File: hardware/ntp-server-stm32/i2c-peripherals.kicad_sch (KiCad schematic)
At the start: 13 parts, among them U57 TMP117xxDRV, U58 TMP117xxDRV, U59 LIS2DH12TR, U60 ATECC608B-SSHDA, U61 IIS2MDCTR

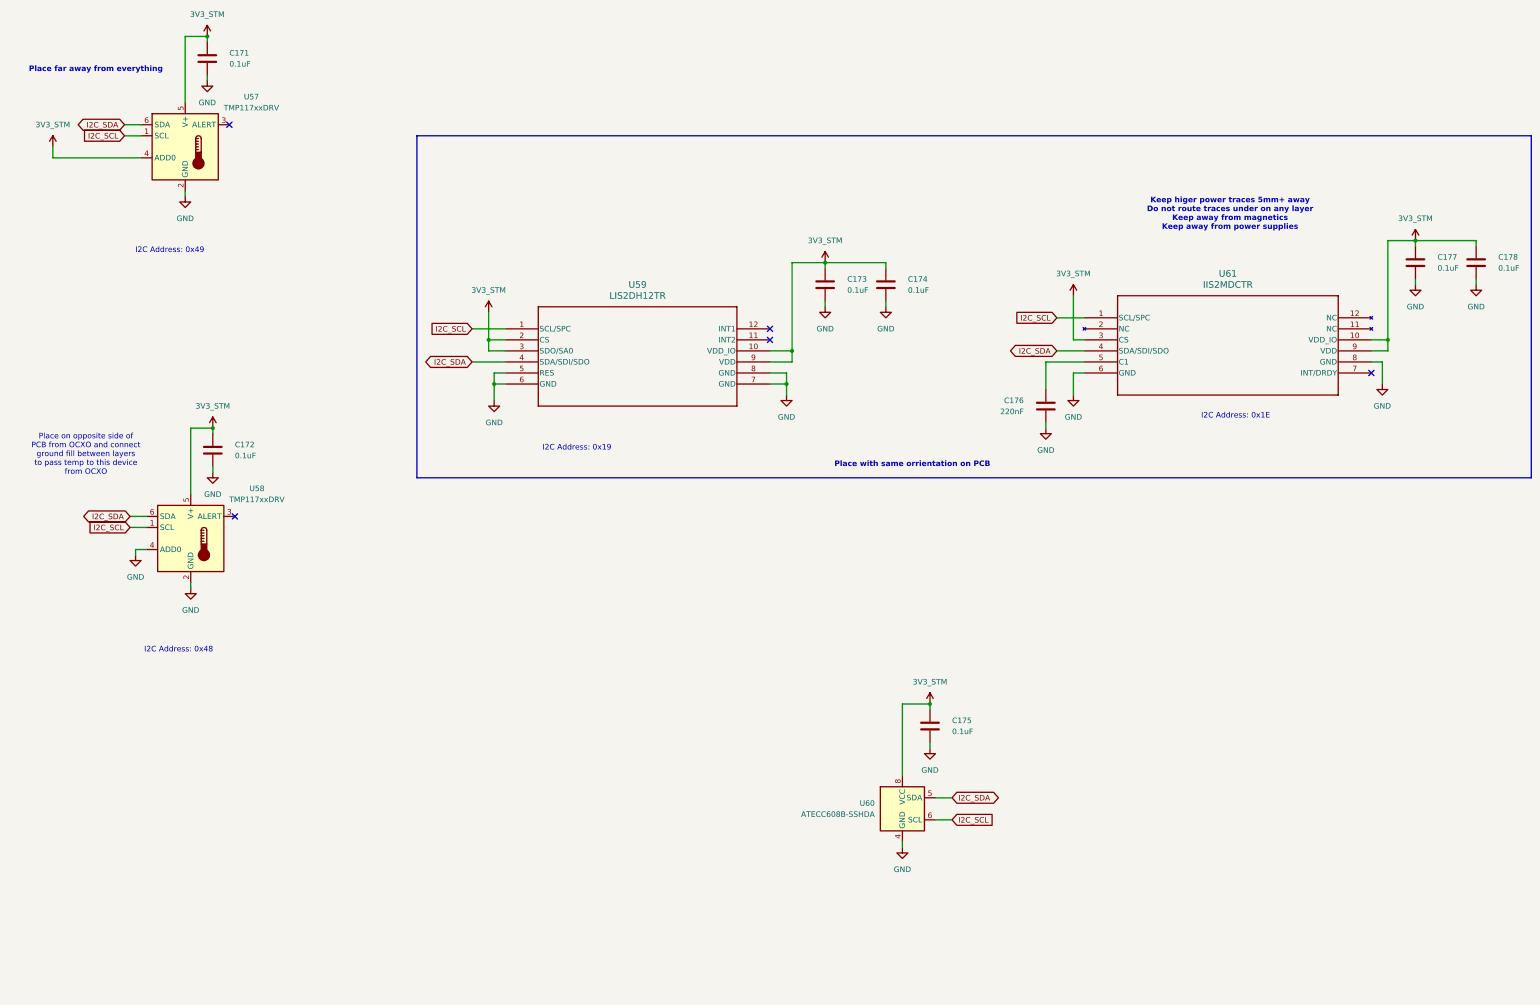
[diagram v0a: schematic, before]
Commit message: Updates
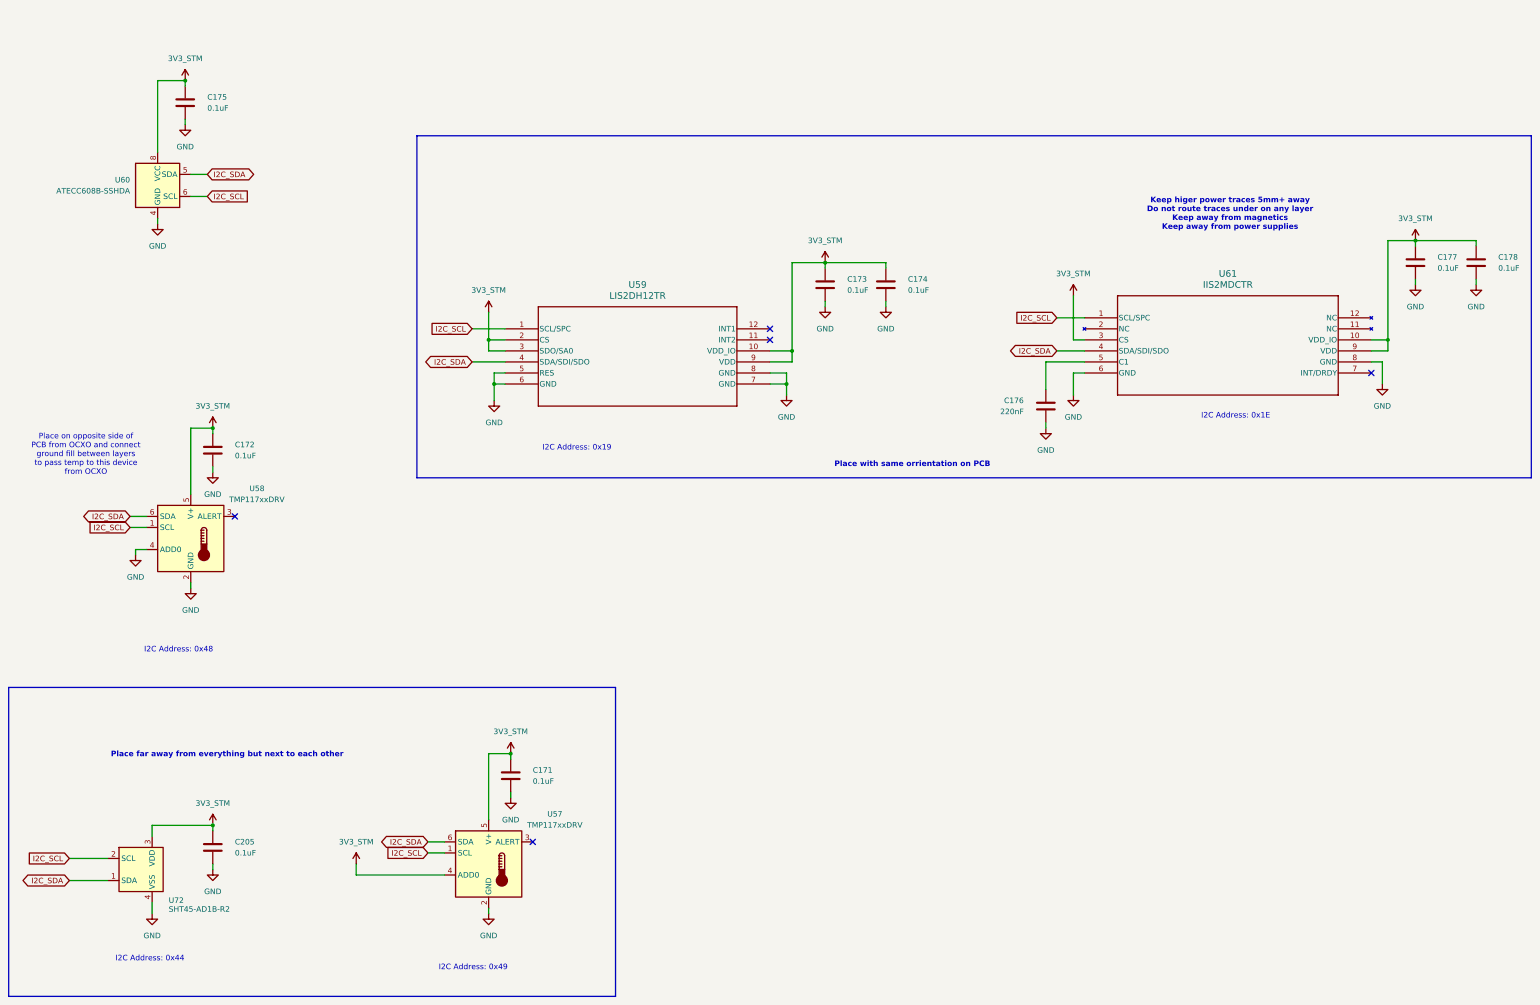
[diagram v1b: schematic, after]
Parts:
- added C205: 0.1uF, 0402 (1005 Metric), symbol Device:C
- added U72: SHT45-AD1B-R2, Sensor_Humidity:Sensirion_DFN-4_1.5x1.5mm_P0.8mm_SHT4x_NoCentralPad, symbol Sensor_Humidity:SHT4x
- C171, C172, C173, C174, C175, C177, C178: footprint C_0402_1005Metric -> 0402 (1005 Metric); DIELECTRIC (none) -> X7R; DIGIKEY_PART_NUMBER 490-6328-2-ND -> 490-4759-1-ND; MANUFACTURER_PART_NUMBER GRM155R71C104KA88J -> GCM155R71C104KA55D; TOLERANCE (none) -> 10%; VOLTAGE (none) -> 16V
- C176: footprint C_0402_1005Metric -> 0402 (1005 Metric); DIELECTRIC (none) -> X7R; DIGIKEY_PART_NUMBER 445-5972-1-ND -> 490-GCM155R71C224KE02JCT-ND; MANUFACTURER TDK -> Murata; MANUFACTURER_PART_NUMBER C2012X7R1E475K125AB -> GCM155R71C224KE02J; TOLERANCE (none) -> 10%; VOLTAGE (none) -> 16V
- U57, U58: MANUFACTURER (none) -> Texas Instruments; MANUFACTURER_PART_NUMBER TMP117xxDRV -> TMP117AIDRVR
- U59, U61: MANUFACTURER (none) -> STMicroelectronics
- U60: MANUFACTURER (none) -> Microchip
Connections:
- net 3V3_STM: now also C205.1, U72.3 (VDD)
- net GND: now also C205.2, U72.4 (VSS)
- net I2C_SCL: now also U72.2 (SCL)
- net I2C_SDA: now also U72.1 (SDA)
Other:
- note added: "I2C Address: 0x44"
- note added: "Place far away from everything but next to each other"
- note removed: "Place far away from everything"
- moved on the sheet: C171, C175, U57, U60

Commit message: Bom updates
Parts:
- U57, U58: DIGIKEY_PART_NUMBER (none) -> 296-51834-1-ND
- U59: DIGIKEY_PART_NUMBER (none) -> 497-14851-1-ND
- U60: DIGIKEY_PART_NUMBER (none) -> 150-ATECC608B-SSHDA-TCT-ND
- U61: DIGIKEY_PART_NUMBER (none) -> 497-17728-1-ND
- U72: DIGIKEY_PART_NUMBER (none) -> 1649-SHT45-AD1B-R2CT-ND
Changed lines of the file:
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@@
+			)
+		)
+		(property "DIGIKEY_PART_NUMBER" "296-51834-1-ND"
+			(at 148.59 224.79 0)
+			(hide yes)
+			(show_name no)
+			(do_not_autoplace no)
+			(effects
+				(font
+					(size 1.27 1.27)
+				)
 			)
 		)
@@
 			)
 		)
+		(property "DIGIKEY_PART_NUMBER" "497-14851-1-ND"
+			(at 152.4 101.6 0)
+			(hide yes)
+			(show_name no)
+			(do_not_autoplace no)
+			(effects
+				(font
+					(size 1.27 1.27)
+				)
+			)
+		)
 		(pin "1"
 		)
@@
 			)
 		)
+		(property "DIGIKEY_PART_NUMBER" "1649-SHT45-AD1B-R2CT-ND"
+			(at 68.58 226.06 0)
+			(hide yes)
+			(show_name no)
+			(do_not_autoplace no)
+			(effects
+				(font
+					(size 1.27 1.27)
+				)
+			)
+		)
 		(pin "2"
 		)
@@
 			)
 		)
+		(property "DIGIKEY_PART_NUMBER" "497-17728-1-ND"
+			(at 285.75 99.06 0)
+			(hide yes)
+			(show_name no)
+			(do_not_autoplace no)
+			(effects
+				(font
+					(size 1.27 1.27)
+				)
+			)
+		)
 		(pin "4"
 		)
@@
 			)
 		)
+		(property "DIGIKEY_PART_NUMBER" "150-ATECC608B-SSHDA-TCT-ND"
+			(at 72.39 68.58 0)
+			(hide yes)
+			(show_name no)
+			(do_not_autoplace no)
+			(effects
+				(font
+					(size 1.27 1.27)
+				)
+			)
+		)
 		(pin "5"
 		)
@@
 			(hide yes)
 			(show_name no)
+			(do_not_autoplace no)
+			(effects
+				(font
+					(size 1.27 1.27)
+				)
+			)
+		)
+		(property "DIGIKEY_PART_NUMBER" "296-51834-1-ND"
+			(at 80.01 149.86 0)
+			(hide yes)
+			(show_name no)

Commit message: Bom updates
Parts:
- U59: footprint LGA-12_STM -> sts1000:LGA-12_STM
- U61: footprint LGA-12_2X2X0P7_STM -> sts1000:LGA-12_2X2X0P7_STM
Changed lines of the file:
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@@
 			)
 		)
-		(property "Footprint" "LGA-12_STM"
+		(property "Footprint" "sts1000:LGA-12_STM"
 			(at 152.4 101.6 0)
 			(hide yes)
@@
 			)
 		)
-		(property "Footprint" "LGA-12_2X2X0P7_STM"
+		(property "Footprint" "sts1000:LGA-12_2X2X0P7_STM"
 			(at 285.75 99.06 0)
 			(hide yes)

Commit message: Add files via upload
Updated, completed placement
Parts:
- C171, C172, C173, C174, C175, C176, C177, C178, C205: footprint 0402 (1005 Metric) -> copy_ref:C_0402_1005Metric
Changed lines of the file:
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@@
 			)
 		)
-		(property "Footprint" "0402 (1005 Metric)"
+		(property "Footprint" "copy_ref:C_0402_1005Metric"
 			(at 86.0552 224.79 0)
 			(hide yes)
@@
 			)
 		)
-		(property "Footprint" "0402 (1005 Metric)"
+		(property "Footprint" "copy_ref:C_0402_1005Metric"
 			(at 227.0252 95.25 0)
 			(hide yes)
@@
 			)
 		)
-		(property "Footprint" "0402 (1005 Metric)"
+		(property "Footprint" "copy_ref:C_0402_1005Metric"
 			(at 86.0552 133.35 0)
 			(hide yes)
@@
 			)
 		)
-		(property "Footprint" "0402 (1005 Metric)"
+		(property "Footprint" "copy_ref:C_0402_1005Metric"
 			(at 275.8948 123.19 0)
 			(hide yes)
@@
 			)
 		)
-		(property "Footprint" "0402 (1005 Metric)"
+		(property "Footprint" "copy_ref:C_0402_1005Metric"
 			(at 362.9152 90.17 0)
 			(hide yes)
@@
 			)
 		)
-		(property "Footprint" "0402 (1005 Metric)"
+		(property "Footprint" "copy_ref:C_0402_1005Metric"
 			(at 376.8852 90.17 0)
 			(hide yes)
@@
 			)
 		)
-		(property "Footprint" "0402 (1005 Metric)"
+		(property "Footprint" "copy_ref:C_0402_1005Metric"
 			(at 240.9952 95.25 0)
 			(hide yes)
@@
 			)
 		)
-		(property "Footprint" "0402 (1005 Metric)"
+		(property "Footprint" "copy_ref:C_0402_1005Metric"
 			(at 79.7052 53.34 0)
 			(hide yes)
@@
 			)
 		)
-		(property "Footprint" "0402 (1005 Metric)"
+		(property "Footprint" "copy_ref:C_0402_1005Metric"
 			(at 154.6352 208.28 0)
 			(hide yes)
